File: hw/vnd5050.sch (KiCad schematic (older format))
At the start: 8 parts, among them U301 VND5050AJTR-E

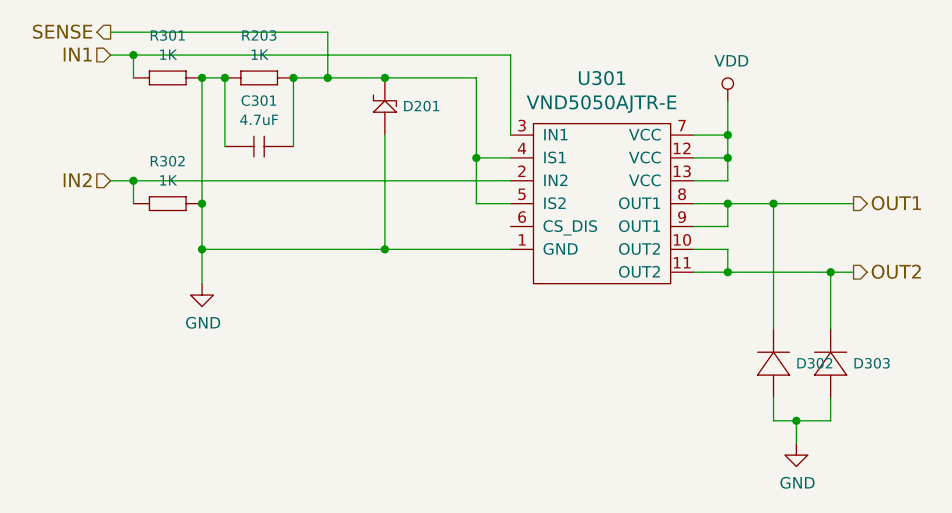
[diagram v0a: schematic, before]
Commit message: pcb 1.3.0 created
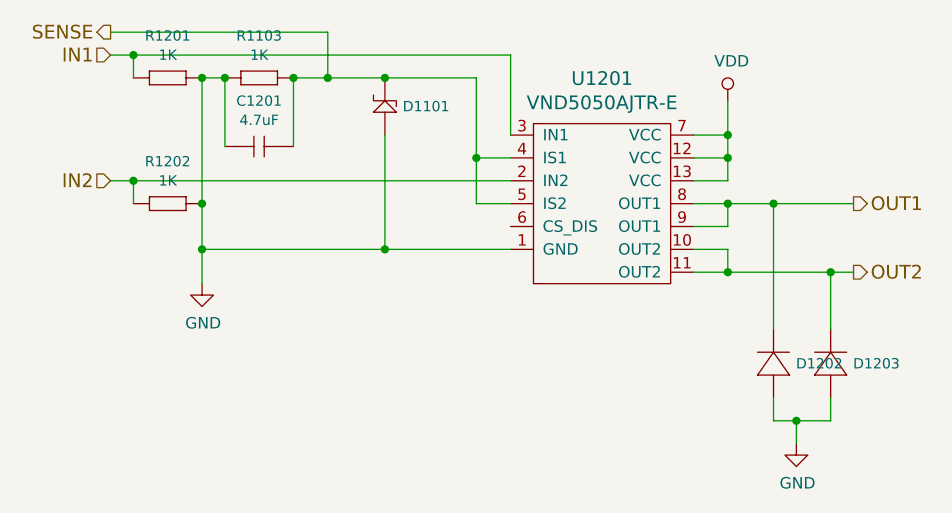
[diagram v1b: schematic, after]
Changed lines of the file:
@@
 AR Path="/5A8DEA06/59D8088A" Ref="U1101"  Part="1"
 AR Path="/5A8DF701/59D8088A" Ref="U1201"  Part="1"
-F 0 "U301" H 4700 4447 60  0000 C CNN
+F 0 "U1201" H 4700 4447 60  0000 C CNN
 F 1 "VND5050AJTR-E" H 4700 4341 60  0000 C CNN
 F 2 "usevolt:PowerSSO-12" H 4600 4400 60  0001 C CNN
@@
 AR Path="/5A8DEA06/59D808C7" Ref="#PWR01103"  Part="1"
 AR Path="/5A8DF701/59D808C7" Ref="#PWR01203"  Part="1"
-F 0 "#PWR0303" H 5250 3500 50  0001 C CNN
+F 0 "#PWR01203" H 5250 3500 50  0001 C CNN
 F 1 "VDD" H 5267 3823 50  0000 C CNN
 F 2 "" H 5250 3650 50  0000 C CNN
@@
 AR Path="/5A8DEA06/59D86DC2" Ref="#PWR01101"  Part="1"
 AR Path="/5A8DF701/59D86DC2" Ref="#PWR01201"  Part="1"
-F 0 "#PWR0301" H 2950 4200 50  0001 C CNN
+F 0 "#PWR01201" H 2950 4200 50  0001 C CNN
 F 1 "GND" H 2955 4277 50  0000 C CNN
 F 2 "" H 2950 4450 50  0000 C CNN
@@
 AR Path="/5A8DEA06/5A05950C" Ref="R1101"  Part="1"
 AR Path="/5A8DF701/5A05950C" Ref="R1201"  Part="1"
-F 0 "R301" H 2800 3734 45  0000 C CNN
+F 0 "R1201" H 2800 3734 45  0000 C CNN
 F 1 "1K" H 2800 3650 45  0000 C CNN
 F 2 "yageo:0603" H 2780 3700 20  0001 C CNN
@@
 AR Path="/5A8DEA06/5A059568" Ref="R1102"  Part="1"
 AR Path="/5A8DF701/5A059568" Ref="R1202"  Part="1"
-F 0 "R302" H 2800 4284 45  0000 C CNN
+F 0 "R1202" H 2800 4284 45  0000 C CNN
 F 1 "1K" H 2800 4200 45  0000 C CNN
 F 2 "yageo:0603" H 2780 4250 20  0001 C CNN
@@
 AR Path="/5A8DEA06/5A2AAF9E" Ref="D1102"  Part="1"
 AR Path="/5A8DF701/5A2AAF9E" Ref="D1202"  Part="1"
-F 0 "D302" V 5400 4652 45  0000 R CNN
+F 0 "D1202" V 5400 4652 45  0000 R CNN
 F 1 "DIODE_RS07J-GS18" H 5470 4690 45  0001 L BNN
 F 2 "usevolt:DO219AB" H 5480 4900 20  0001 C CNN
@@
 AR Path="/5A8DEA06/5A2AB087" Ref="D1103"  Part="1"
 AR Path="/5A8DF701/5A2AB087" Ref="D1203"  Part="1"
-F 0 "D303" V 5650 4652 45  0000 R CNN
+F 0 "D1203" V 5650 4652 45  0000 R CNN
 F 1 "DIODE_RS07J-GS18" H 5720 4690 45  0001 L BNN
 F 2 "usevolt:DO219AB" H 5730 4900 20  0001 C CNN
@@
 AR Path="/5A8DEA06/5A2AB10F" Ref="#PWR01104"  Part="1"
 AR Path="/5A8DF701/5A2AB10F" Ref="#PWR01204"  Part="1"
-F 0 "#PWR0304" H 5550 4900 50  0001 C CNN
+F 0 "#PWR01204" H 5550 4900 50  0001 C CNN
 F 1 "GND" H 5555 4977 50  0000 C CNN
 F 2 "" H 5550 5150 50  0000 C CNN
@@
 AR Path="/5A8DEA06/5A708309" Ref="C1101"  Part="1"
 AR Path="/5A8DF701/5A708309" Ref="C1201"  Part="1"
-F 0 "C301" H 3200 4049 45  0000 C CNN
+F 0 "C1201" H 3200 4049 45  0000 C CNN
 F 1 "4.7uF" H 3200 3965 45  0000 C CNN
 F 2 "kemet:0603" H 3180 4000 20  0001 C CNN
@@
 AR Path="/5A8DEA06/5B6F848F" Ref="R1003"  Part="1"
 AR Path="/5A8DF701/5B6F848F" Ref="R1103"  Part="1"
-F 0 "R203" H 3200 3734 45  0000 C CNN
+F 0 "R1103" H 3200 3734 45  0000 C CNN
 F 1 "1K" H 3200 3650 45  0000 C CNN
 F 2 "yageo:0603" H 3180 3700 20  0001 C CNN
@@
 AR Path="/5A8DEA06/5B701DAD" Ref="D1001"  Part="1"
 AR Path="/5A8DF701/5B701DAD" Ref="D1101"  Part="1"
-F 0 "D201" V 3675 3522 45  0000 R CNN
+F 0 "D1101" V 3675 3522 45  0000 R CNN
 F 1 "ZENER_MM3Z3V6T1G" H 4025 3975 45  0001 L BNN
 F 2 "usevolt:SOD-323" H 3725 3975 20  0001 C CNN
